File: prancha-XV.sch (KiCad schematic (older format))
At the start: 12 parts

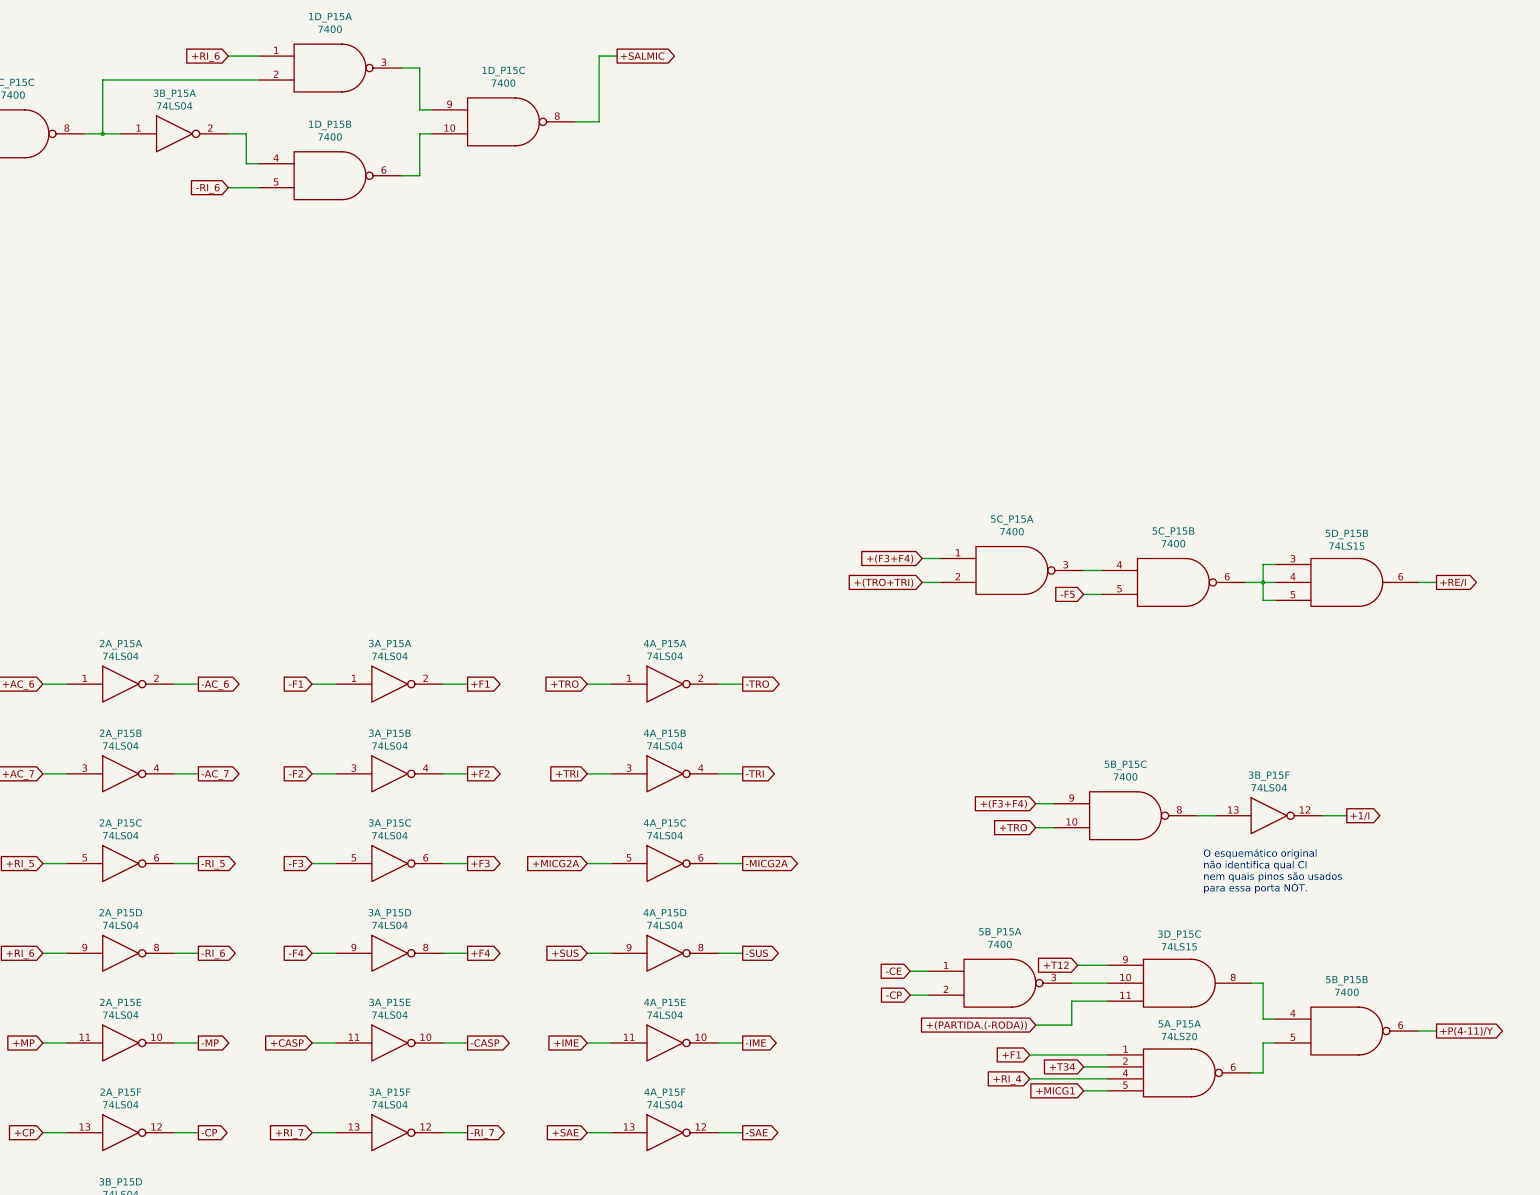
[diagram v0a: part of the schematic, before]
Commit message: mais um trecho da prancha 15
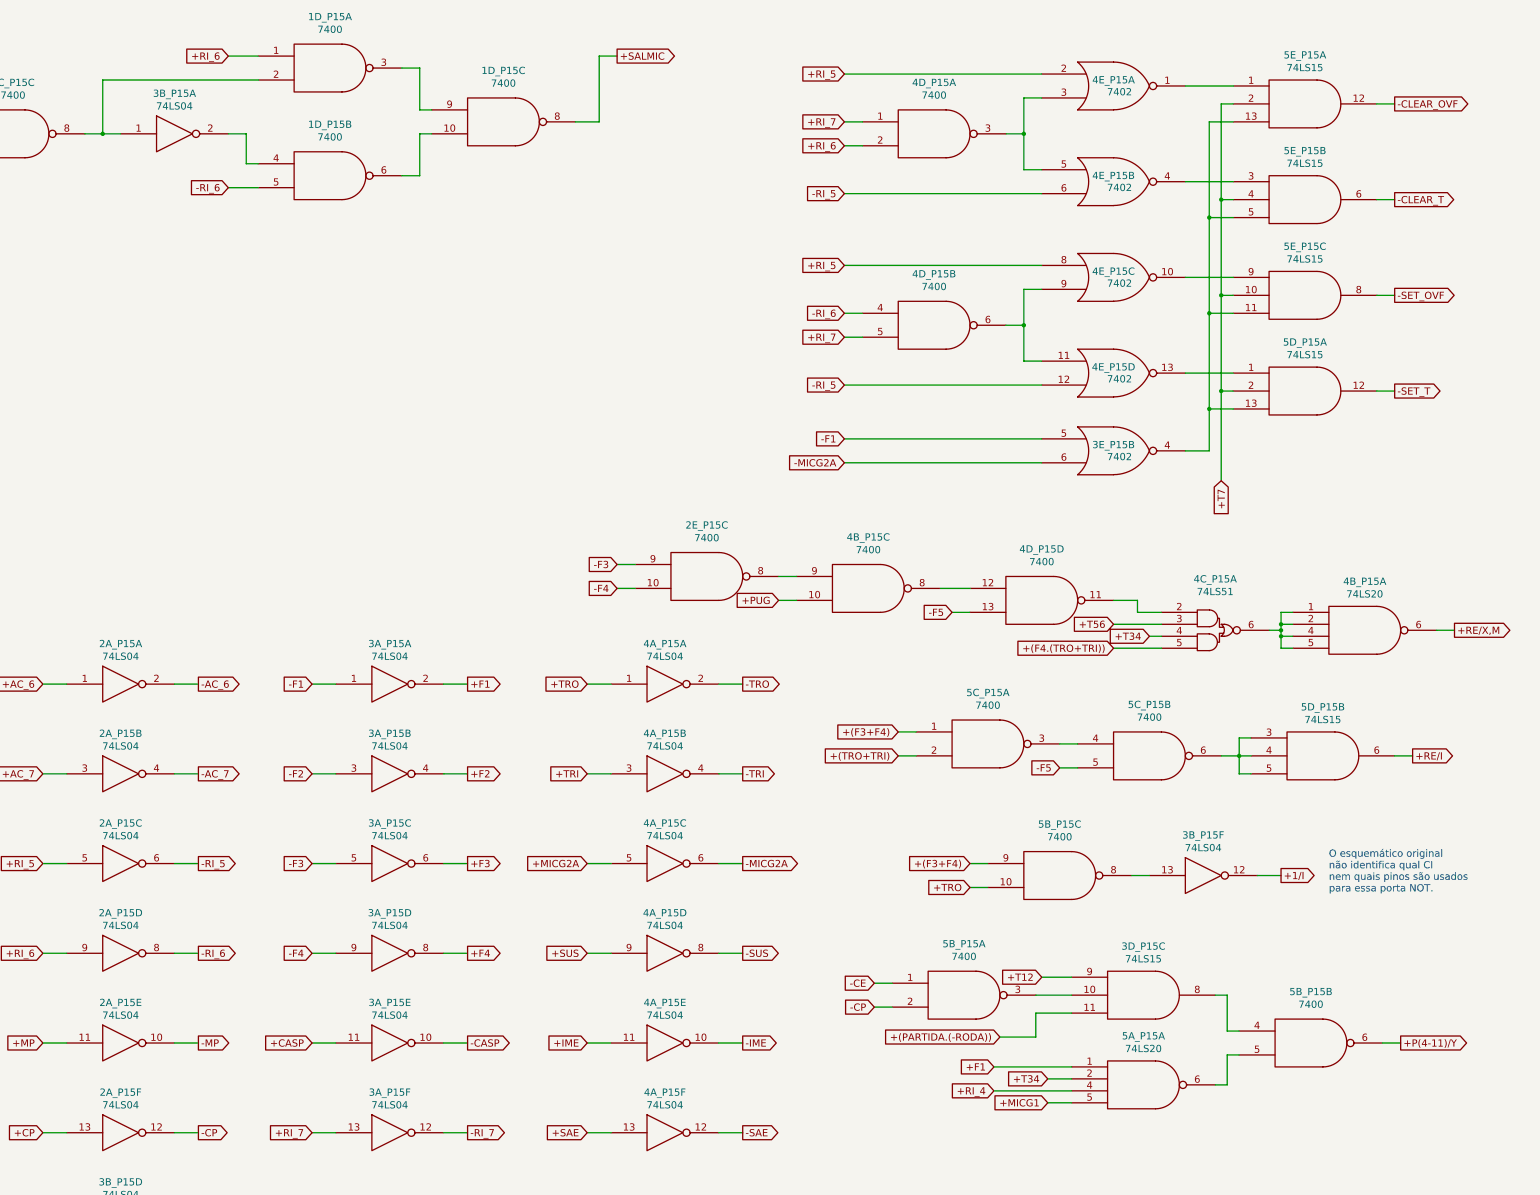
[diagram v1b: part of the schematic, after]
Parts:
- added 2E_P15, 4D_P15: 7400, symbol 7400
- added 3E_P15, 4E_P15: 7402, ~, symbol 7402
- added 4B_P15: 74LS20, symbol 74LS20
- added 4C_P15: 74LS51, symbol 74LS51
- added unit 1 of 5D_P15
- added 5E_P15: 74LS15, symbol 74LS15
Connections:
- net +RI_5: now also 4E_P15.2, 4E_P15.8
- net +RI_6: now also 4D_P15.2
- net +RI_7: now also 4D_P15.1, 4D_P15.5
- net +T34: now also 4C_P15.4
- net -F1: now also 3E_P15.5
- net -F3: now also 2E_P15.9
- net -F4: now also 2E_P15.10
- net -F5: now also 4D_P15.13
- net -MICG2A: now also 3E_P15.6
- net -RI_5: now also 4E_P15.12, 4E_P15.6
- net -RI_6: now also 4D_P15.4
- net GND: now also 2E_P15.7 (GND), 3E_P15.7 (GND), 4B_P15.7 (GND), 4B_P15.7 (GND), 4C_P15.7 (GND), 4D_P15.7 (GND), 4D_P15.7 (GND), 4D_P15.7 (GND), 4E_P15.7 (GND), 4E_P15.7 (GND), 4E_P15.7 (GND), 4E_P15.7 (GND), 5D_P15.7 (GND), 5E_P15.7 (GND), 5E_P15.7 (GND), 5E_P15.7 (GND)
- net VCC: now also 2E_P15.14 (VCC), 3E_P15.14 (VCC), 4B_P15.14 (VCC), 4B_P15.14 (VCC), 4C_P15.14 (VCC), 4D_P15.14 (VCC), 4D_P15.14 (VCC), 4D_P15.14 (VCC), 4E_P15.14 (VCC), 4E_P15.14 (VCC), 4E_P15.14 (VCC), 4E_P15.14 (VCC), 5D_P15.14 (VCC), 5E_P15.14 (VCC), 5E_P15.14 (VCC), 5E_P15.14 (VCC)
- new net: 4B_P15.1, 4B_P15.2, 4B_P15.4, 4B_P15.5, 4C_P15.6
- new net: 4C_P15.2, 4D_P15.11
- new net: 2E_P15.8, 4B_P15.9
- new net: 4B_P15.8, 4D_P15.12
- new net: 4D_P15.6, 4E_P15.11, 4E_P15.9
- new net: 4E_P15.13, 5D_P15.1
- new net: 3E_P15.4, 5D_P15.13, 5E_P15.11, 5E_P15.13, 5E_P15.5
- new net: 4E_P15.10, 5E_P15.9
- new net: 4E_P15.4, 5E_P15.3
- new net: 4D_P15.3, 4E_P15.3, 4E_P15.5
- new net: 4E_P15.1, 5E_P15.1
- new net +(F4.(TRO+TRI)): 4C_P15.5
- new net +PUG: 4B_P15.10
- new net +RE/X,M: 4B_P15.6
- new net +T56: 4C_P15.3
- new net +T7: 5D_P15.2, 5E_P15.10, 5E_P15.2, 5E_P15.4
- new net -CLEAR_OVF: 5E_P15.12
- new net -CLEAR_T: 5E_P15.6
- new net -SET_OVF: 5E_P15.8
- new net -SET_T: 5D_P15.12
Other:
- moved on the sheet: 3B_P15F, 3D_P15C, 5A_P15A, 5B_P15A, 5B_P15B, 5B_P15C, 5C_P15A, 5C_P15B, 5D_P15B
